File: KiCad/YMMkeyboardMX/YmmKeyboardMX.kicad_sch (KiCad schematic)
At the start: 123 parts, among them SW10 SW_Push, SW11 SW_Push, SW12 SW_Push, SW13 SW_Push, SW14 SW_Push, SW15 SW_Push, SW16 SW_Push, SW17 SW_Push, SW18 SW_Push, SW19 SW_Push, SW2 SW_Push, SW20 SW_Push, SW21 SW_Push, SW22 SW_Push, SW23 SW_Push, SW24 SW_Push, SW25 SW_Push, SW26 SW_Push, SW27 SW_Push, SW28 SW_Push, SW29 SW_Push, SW3 SW_Push, SW30 SW_Push, SW31 SW_Push, SW32 RotaryEncoder_Switch, SW4 SW_Push, SW5 SW_Push, SW6 SW_Push, SW7 SW_Push, SW8 SW_Push, SW9 SW_Push, U1 RP2040-Zero

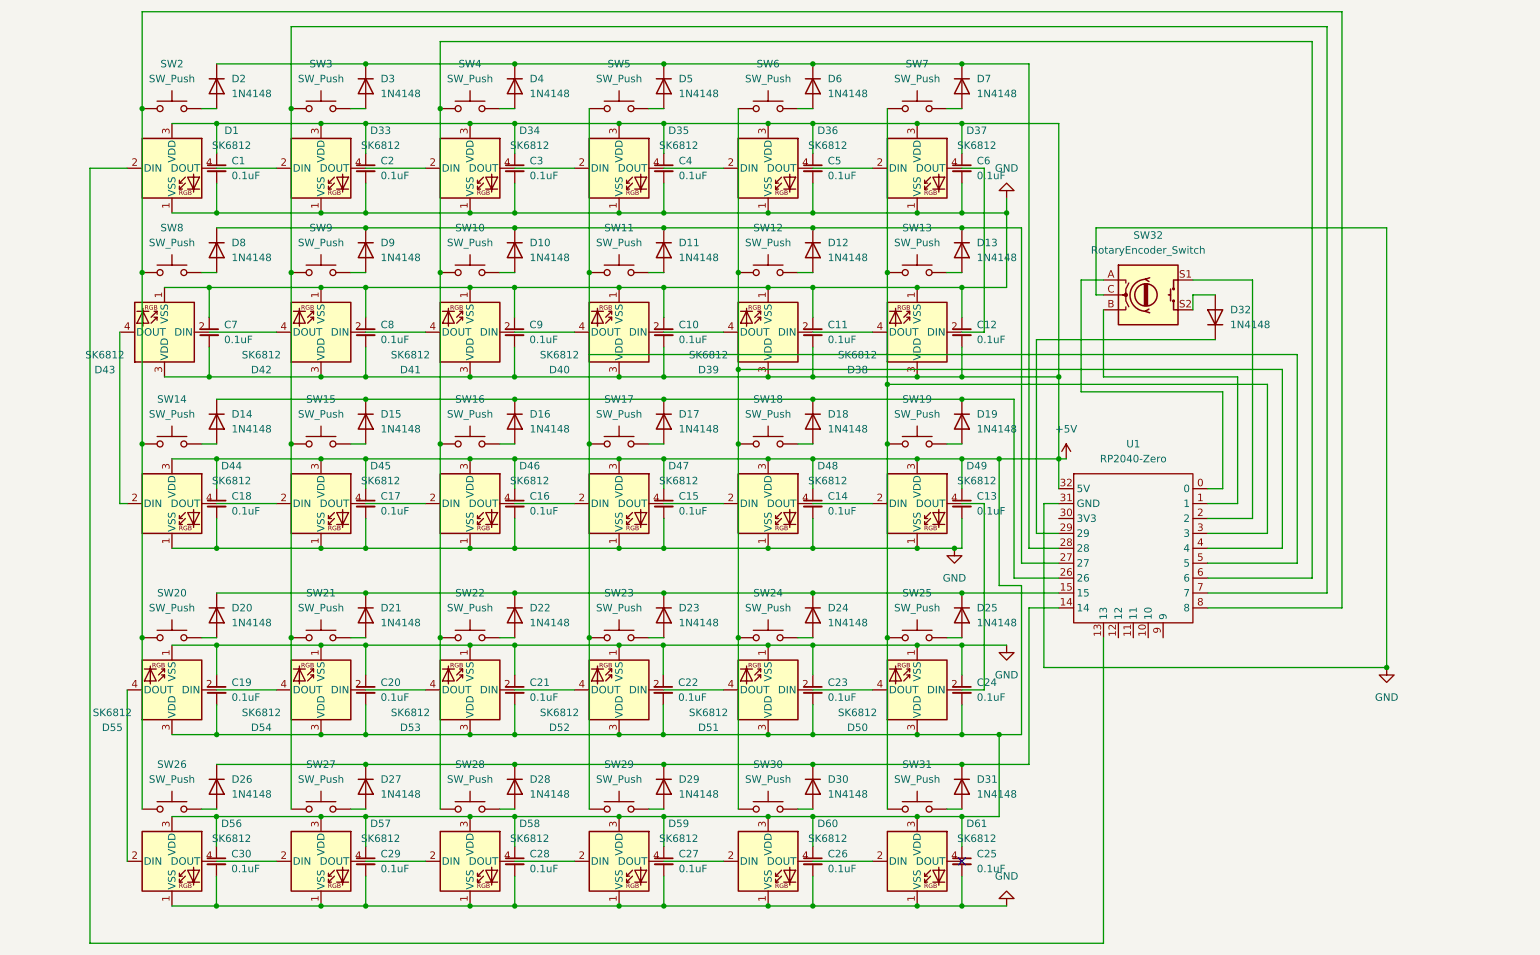
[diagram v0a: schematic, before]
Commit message: 3号機発注
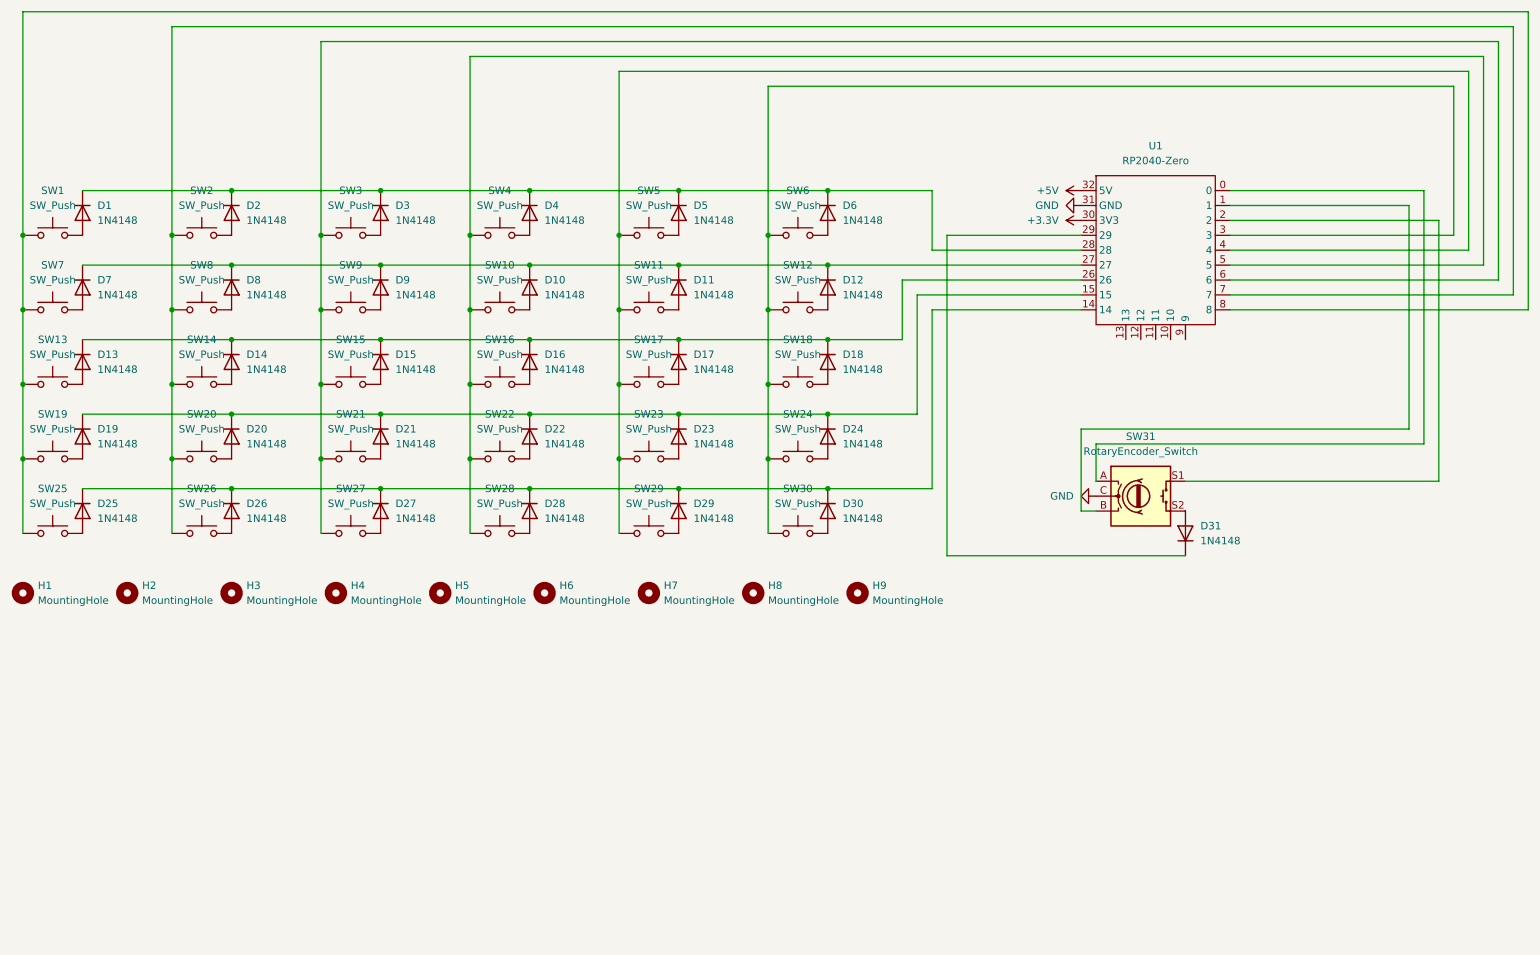
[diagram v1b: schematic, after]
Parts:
- removed C1, C10, C11, C12, C13, C14, C15, C16, C17, C18, C19, C2, C20, C21, C22, C23, C24, C25, C26, C27, C28, C29, C3, C30, C4, C5, C6, C7, C8, C9: 0.1uF, Capacitor_SMD:C_0603_1608Metric_Pad1.08x0.95mm_HandSolder, symbol Device:C_Small
- removed D1, D33, D34, D35, D36, D37, D38, D39, D40, D41, D42, D43, D44, D45, D46, D47, D48, D49, D50, D51, D52, D53, D54, D55, D56, D57, D58, D59, D60, D61: SK6812, LED_SMD:LED_SK6812_PLCC4_5.0x5.0mm_P3.2mm, symbol LED:SK6812
- removed D32: 1N4148, Diode_THT:D_DO-35_SOD27_P7.62mm_Horizontal, symbol Diode:1N4148
- removed SW31: SW_Push, Button_Switch_THT:SW_PUSH_6mm, symbol Switch:SW_Push
- removed SW32: RotaryEncoder_Switch, Rotary_Encoder:RotaryEncoder_Alps_EC11E-Switch_Vertical_H20mm, symbol Device:RotaryEncoder_Switch
- added D1: 1N4148, Diode_SMD:D_SOD-123, symbol Diode:1N4148
- added H1, H2, H3, H4, H5, H6, H7, H8, H9: MountingHole, MountingHole:MountingHole_2.2mm_M2, symbol Mechanical:MountingHole
- added SW1: SW_Push, isw-kbd:CherryMX_Hotswap_1u, symbol Switch:SW_Push
- added SW31: RotaryEncoder_Switch, Rotary_Encoder:RotaryEncoder_Alps_EC11E-Switch_Vertical_H20mm, symbol Device:RotaryEncoder_Switch
- D10, D11, D12, D13, D14, D15, D16, D17, D18, D19, D2, D20, D21, D22, D23, D24, D25, D26, D27, D28, D29, D3, D30, D31, D4, D5, D6, D7, D8, D9: footprint Diode_THT:D_DO-35_SOD27_P7.62mm_Horizontal -> Diode_SMD:D_SOD-123
- SW10, SW11, SW12, SW13, SW14, SW15, SW16, SW17, SW18, SW19, SW2, SW20, SW21, SW22, SW23, SW24, SW25, SW26, SW27, SW28, SW29, SW3, SW30, SW4, SW5, SW6, SW7, SW8, SW9: footprint Button_Switch_THT:SW_PUSH_6mm -> isw-kbd:CherryMX_Hotswap_1u
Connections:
- net GND: now also SW31.C
- net at U1.0: now also SW31.A
- net at U1.1: now also SW31.B
- net at D26.1 (K), D27.1 (K), D28.1 (K)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: now also D25.1 (K); no longer D31.1 (K)
- net at D20.1 (K), D21.1 (K), D22.1 (K)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: now also D19.1 (K); no longer D25.1 (K)
- net at U1.2: now also SW31.S1
- net at D14.1 (K), D15.1 (K), D16.1 (K)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: now also D13.1 (K); no longer D19.1 (K)
- net at D10.1 (K), D11.1 (K), D12.1 (K)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: now also D7.1 (K); no longer D13.1 (K)
- net at D2.1 (K), D3.1 (K), D4.1 (K)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: now also D1.1 (K); no longer D7.1 (K)
- net at U1.29: now also D31.1 (K)
- net at SW13.1, SW19.1, SW25.1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: now also U1.8, SW1.1; no longer U1.3
- net +3.3V: now reaches U1.30 (3V3)
- net at SW12.1, SW18.1, SW24.1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: now also U1.3; no longer U1.4
- net at SW11.1, SW17.1, SW23.1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: now also U1.4; no longer U1.5
- net at SW10.1, SW16.1, SW22.1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: now also U1.5; no longer U1.6
- net at SW15.1, SW21.1, SW27.1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: now also U1.6; no longer U1.7
- net at SW14.1, SW2.1, SW20.1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: now also U1.7; no longer U1.8
- net at D31.2 (A): now also SW31.S2
- new net: D1.2 (A), SW1.2
- no-connect marks 1 -> 0
